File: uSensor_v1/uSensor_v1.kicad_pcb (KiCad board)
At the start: 2 copper layers, 145.5 x 81.4 mm, 287 parts, among them J1 +12V Supply, J2 Conn_01x03, J3 Conn_01x03, J4 NS25-W8P 6-pin 2,54mm, J5 USB_B, J6 GNDA-GNDD Jumper, J7 Barrel_Jack_Switch, Q1 BC817-25, Q2 BC817-25, Q3 BC847PN-7-F, Q4 BC847PN-7-F, SW1 SW_Push, SW2 SW_Push, SW3 SW_Push, U1 AM10TW-2405DZ, U10 KSS-213 Connector, U11 AD7795, U12 AD5667, U13 TBD, U14 TBD, U15 REF192, U16 TBD, U17 TBD, U2 LD1117A, U22 RCLAMP, U3 STM32F407VGTx, U4 MCP9700AT, U5 MCP9700AT, U6 LM6132A, U7 MCP9700AT, U8 MCP9700AT, U9 UG-2864KSWLG01

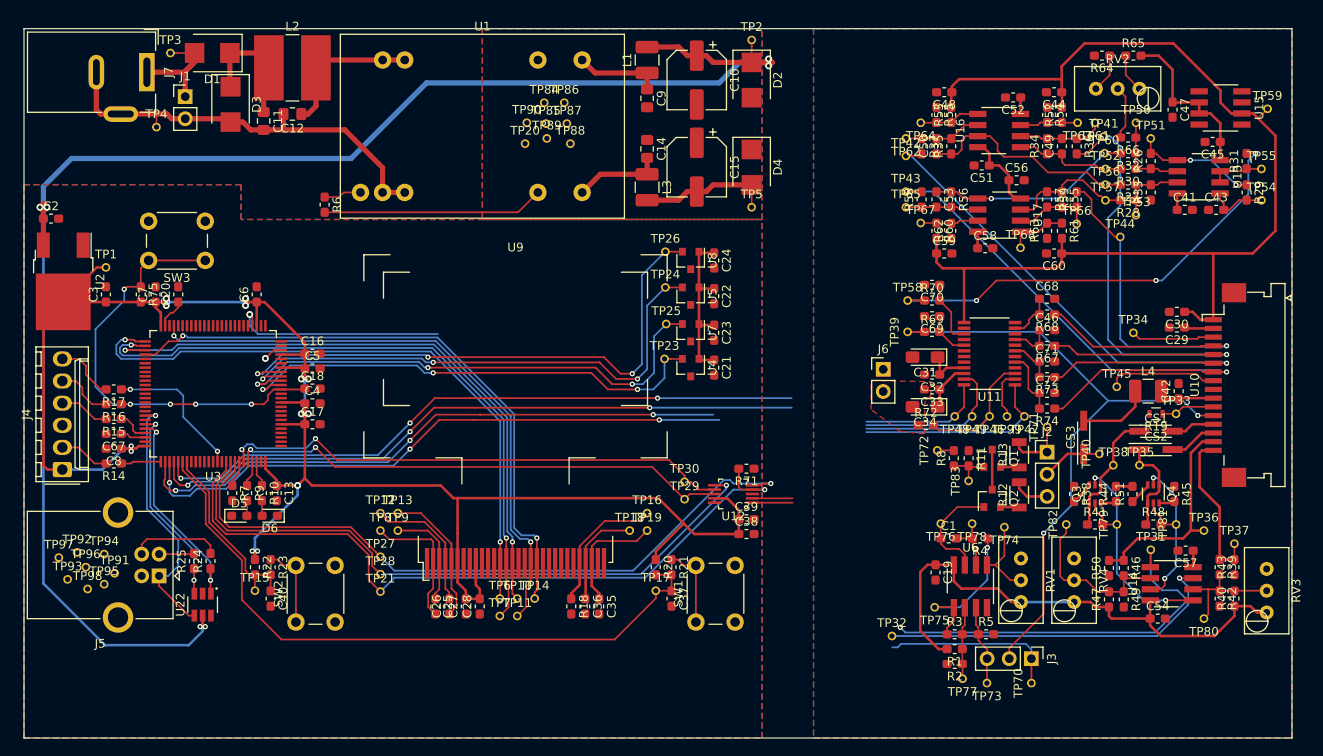
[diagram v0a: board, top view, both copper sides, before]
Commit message: Layout in progress.
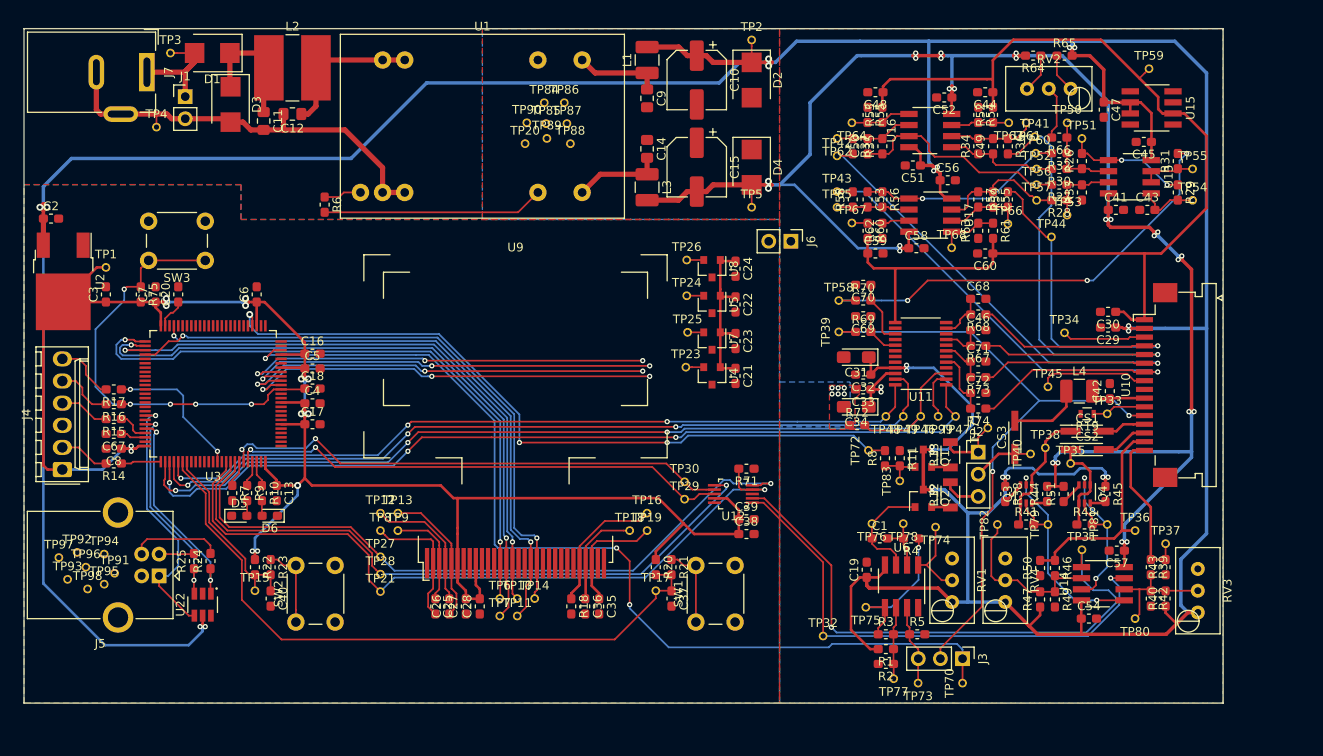
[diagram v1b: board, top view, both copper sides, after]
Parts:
- moved J6 18.1 mm to (101.0, 37.4), turned to 270 degrees
- moved TP59 14.4 mm to (142.1, 17.6)
- moved TP38 8.05 mm to (130.2, 61.1)
- moved C19 7.91 mm to (109.7, 75.1), turned to 90 degrees
- moved TP35 7.90 mm to (133.1, 62.9)
- moved C29 7.90 mm to (137.4, 47.3)
- moved C30 7.90 mm to (137.4, 45.5)
- moved C31 7.90 mm to (108.5, 50.7)
- moved C32 7.90 mm to (109.3, 52.7)
- moved C33 7.90 mm to (109.3, 54.4)
- moved C34 7.90 mm to (108.5, 56.4)
- moved C42 7.90 mm to (137.6, 54.6)
- moved C43 7.90 mm to (141.9, 33.8)
- moved C45 7.90 mm to (141.5, 26.0)
- moved C46 7.90 mm to (122.5, 47.6)
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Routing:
- net +5V: track 295.3 -> 525.7 mm, vias 6 -> 22
- net -5V: track 24.8 -> 220.5 mm, vias 0 -> 24
- net SENS_PD_ADC: track 22.4 -> 112.0 mm, vias 1 -> 3
- net DAC_LD_CTRL: track 26.6 -> 84.1 mm, vias 1 -> 3
- net TEMP_SENS_OUT_4: track 65.1 -> 49.8 mm
- net DAC_OUT_COIL_F_CTRL: track 45.1 -> 59.9 mm
- net DAC_OUT_COIL_T_CTRL: track 49.7 -> 64.4 mm
- net TEMP_SENS_OUT_3: track 60.9 -> 49.6 mm
- net ADC_~CS: track 98.5 -> 107.5 mm
- net TEMP_SENS_OUT_2: track 59.0 -> 50.1 mm
- net ADC_SCLK: track 93.3 -> 101.7 mm
- net TEMP_SENS_OUT_1: track 55.5 -> 50.1 mm
- net +3V3: track 246.1 -> 249.9 mm, vias 13 -> 15
- net REF_2.5V: track 127.0 -> 126.2 mm
- net GNDD: vias 0 -> 6
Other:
- board size 145.5 x 81.4 mm -> 137.6 x 77.4 mm
